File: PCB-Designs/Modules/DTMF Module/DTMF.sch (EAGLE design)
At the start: 18 parts, among them IC1 CM8870CP

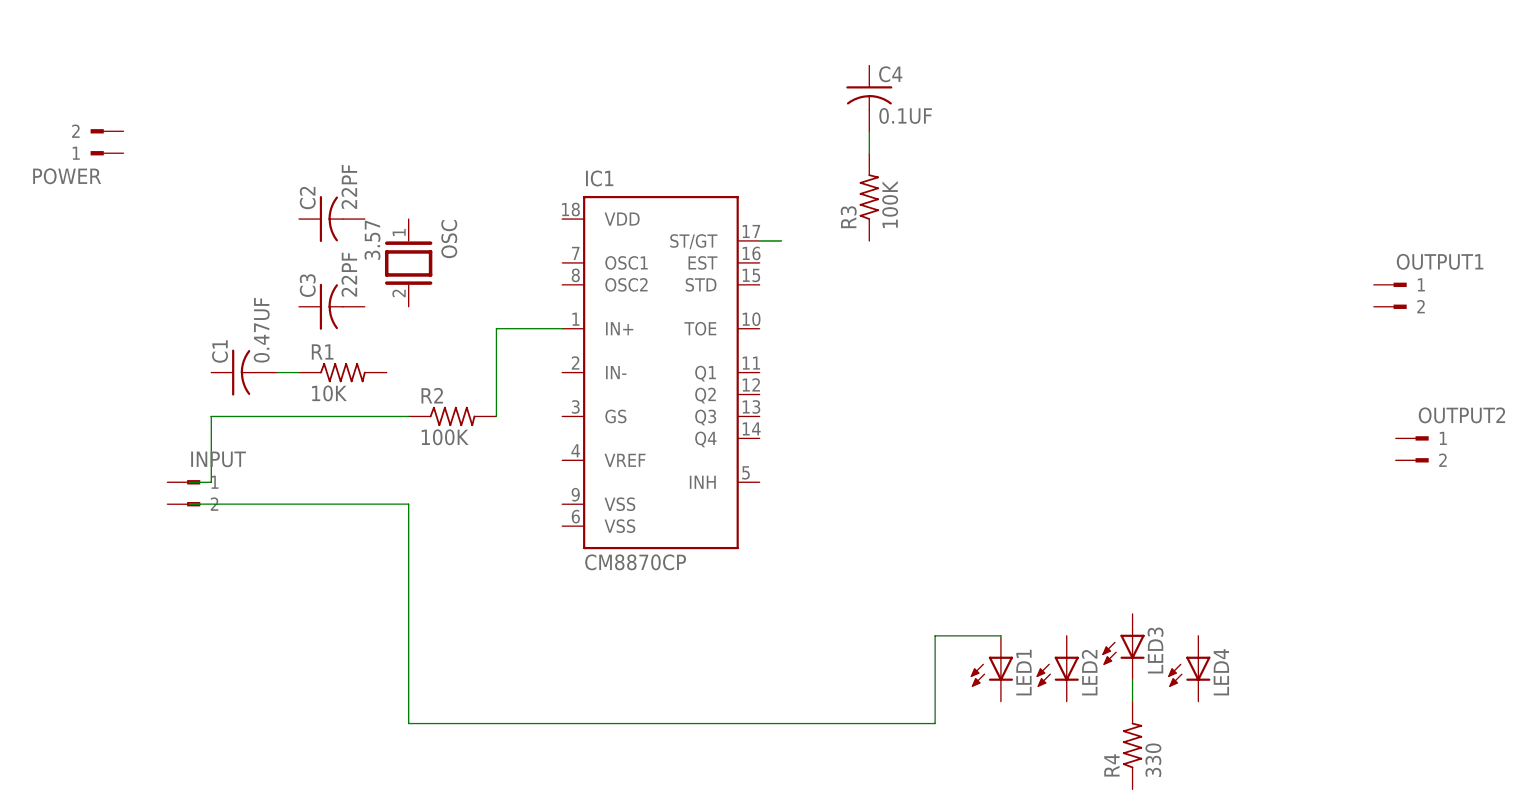
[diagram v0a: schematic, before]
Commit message: change
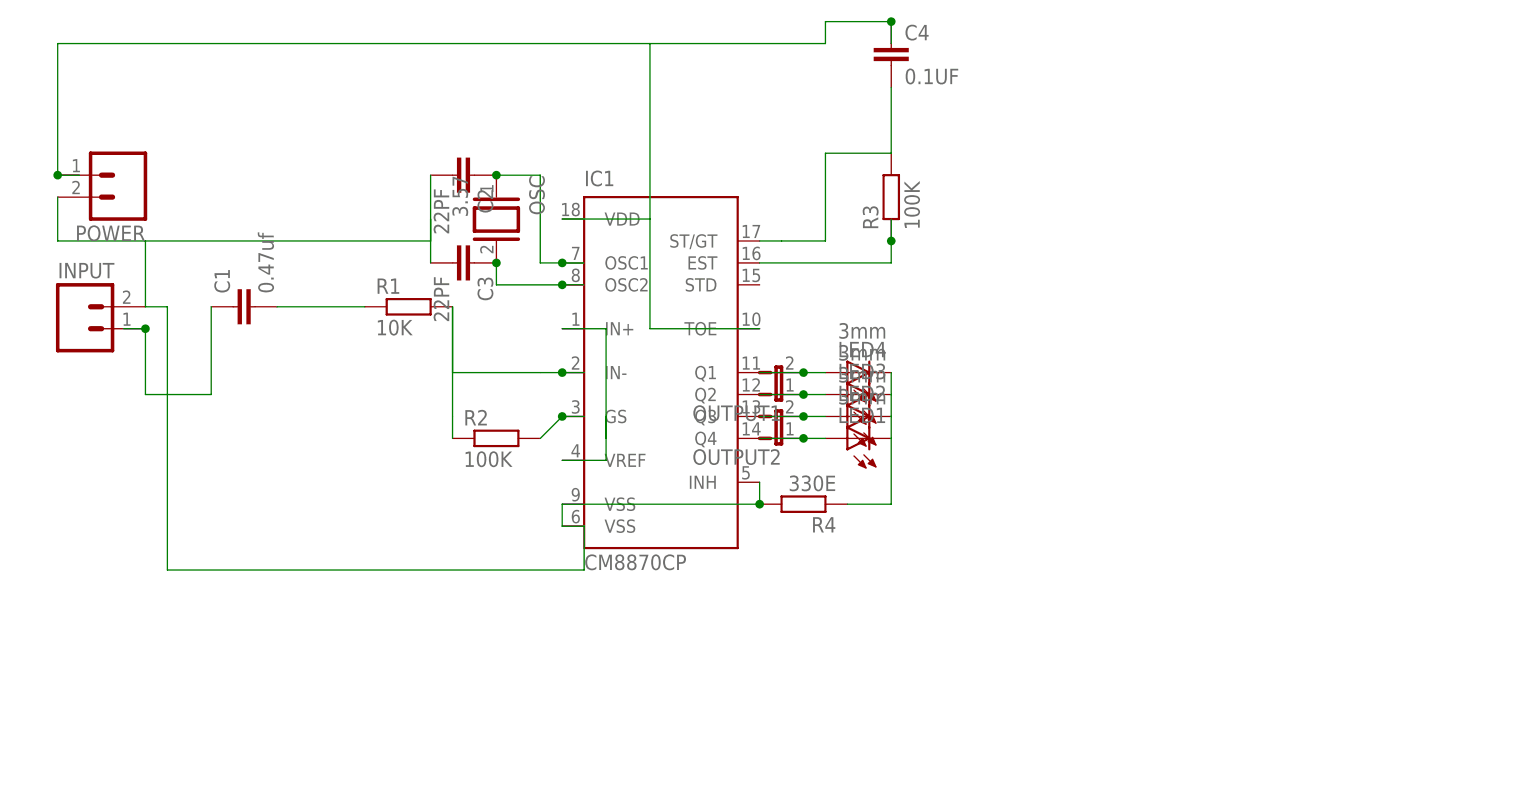
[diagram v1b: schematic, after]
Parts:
- C1: value 0.47UF -> 0.47uf; device resistor:C-US050-024X044 -> capacitor-wima:C2.5/2
- C2, C3, C4: device resistor:C-US050-024X044 -> capacitor-wima:C2.5/2
- INPUT, POWER: device con-weidmueller-sl35:180-2 -> con-amp-quick:M02
- LED1, LED2, LED3, LED4: value (none) -> 3mm; device led:LEDSQR2X5 -> led:LED3MM
- OUTPUT1, OUTPUT2: device con-weidmueller-sl35:180-2 -> jumper:JP1E
- R1, R2, R3: device rcl:R-US_VMTB60 -> rcl:R-EU_0204/7
- R4: value 330 -> 330E; device rcl:R-US_VMTB60 -> rcl:R-EU_0204/7
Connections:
- removed net N$16: LED3.C, R4.2
- removed net N$9: C4.2, R3.2
- new net N$10: C4.1, IC1.TOE, IC1.VDD, POWER.1
- new net N$11: C1.1, INPUT.1
- new net N$12: IC1.IN-, R1.2, R2.1
- new net N$13: IC1.IN+, IC1.VREF
- new net N$14: C2.1, IC1.OSC1, OSC.1
- new net N$15: C3.1, IC1.OSC2, OSC.2
- new net N$17: IC1.EST, R3.1
- new net N$5: IC1.Q1, LED4.A, OUTPUT1.2
- new net N$6: IC1.Q2, LED3.A, OUTPUT1.1
- new net N$7: IC1.Q3, LED2.A, OUTPUT2.2
- new net N$8: IC1.Q4, LED1.A, OUTPUT2.1
- net N$1: now also C2.2, C3.2, IC1.INH, IC1.VSS, IC1.VSS@1, INPUT.2, POWER.2, R4.2; no longer R2.1
- net N$24: now also C4.2, R3.2
- net N$3: now also IC1.GS; no longer IC1.IN+
- net N$4: now also LED1.C, LED2.C, LED3.C, LED4.C, R4.1; no longer LED1.A
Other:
- moved on the sheet: C1, C2, C3, C4, LED1, LED2, LED3, LED4, OSC
